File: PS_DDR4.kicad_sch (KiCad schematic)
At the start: 4 parts, among them U12 K4A8G165WC-BCTD, U14 K4A8G165WC-BCTD

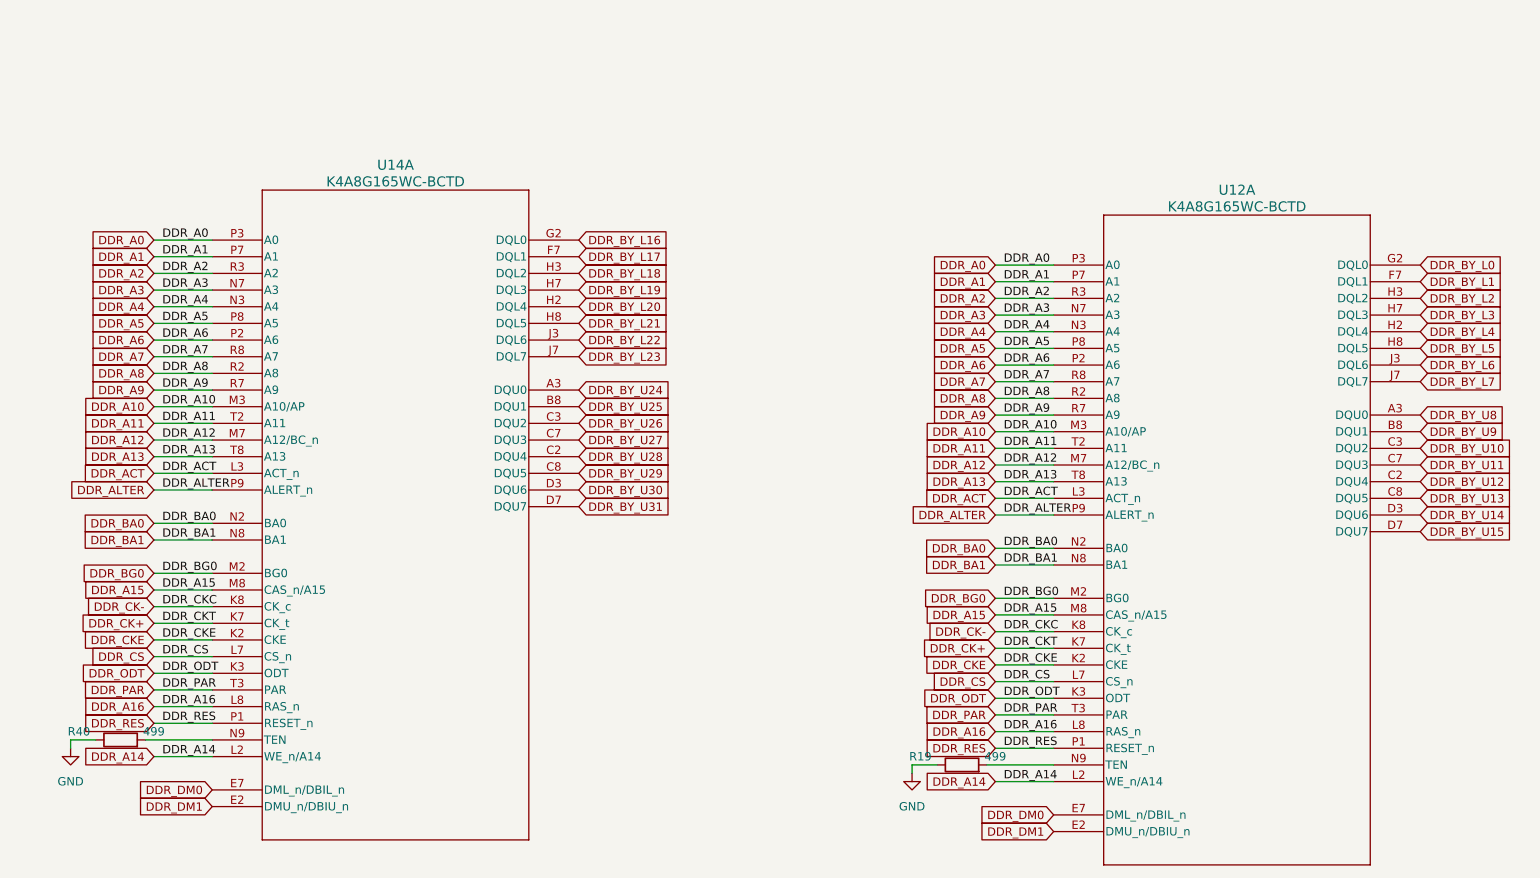
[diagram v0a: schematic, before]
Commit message: DDR4 finish
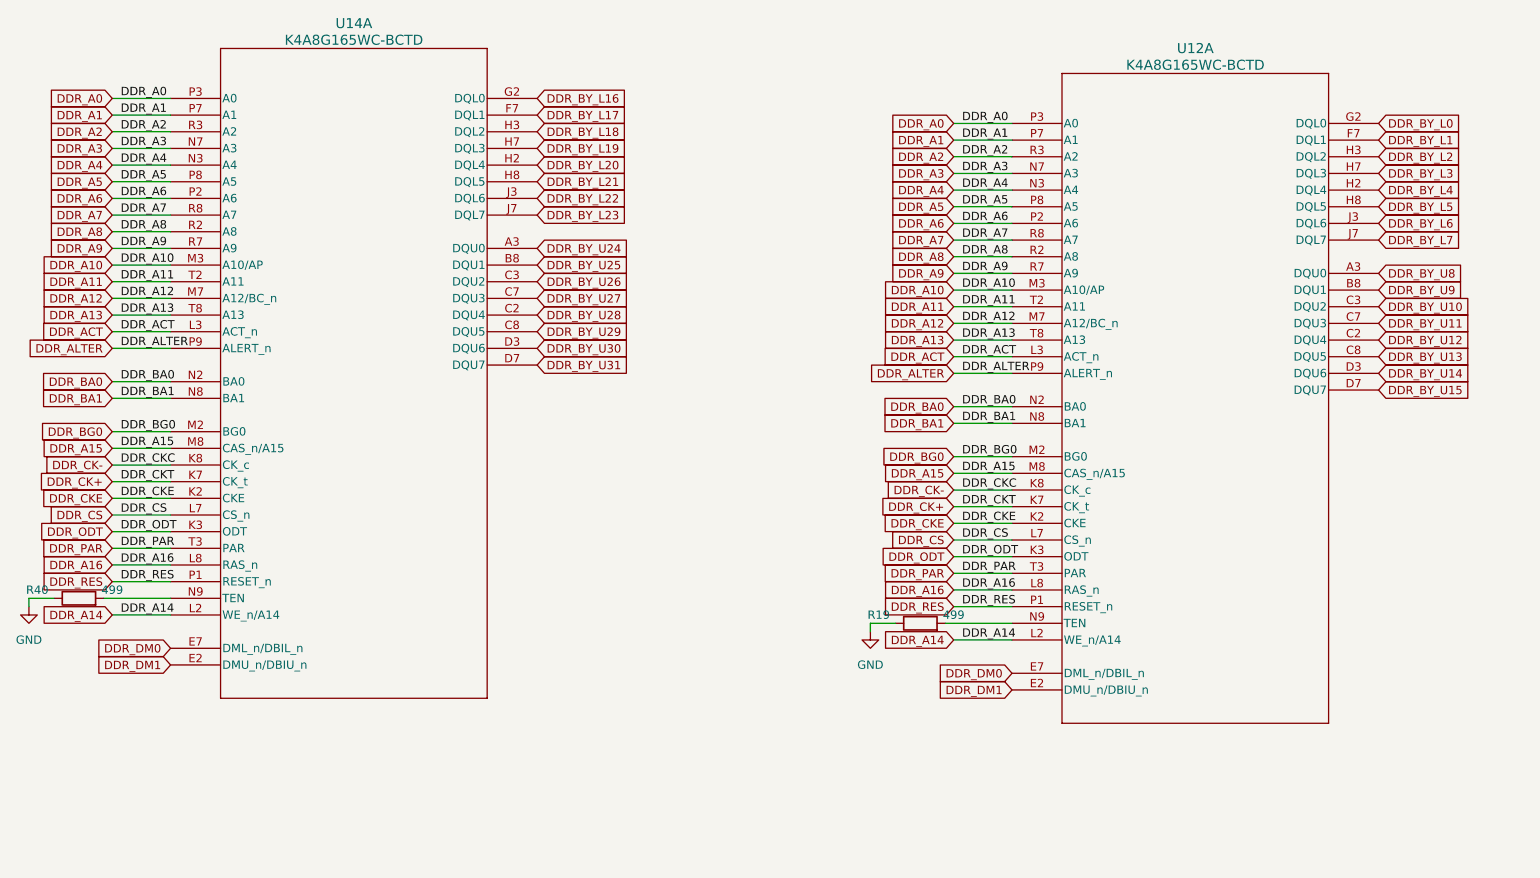
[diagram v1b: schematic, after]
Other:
- moved on the sheet: R19, R40, U12A, U14A
